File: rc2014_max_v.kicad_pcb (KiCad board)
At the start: 4 copper layers, 101.6 x 50.8 mm, 128 parts, among them J1 M3 Mounting Hole, J2 Conn_01x40, J3 Conn_01x24, J4 USB_B_Micro, J5 AVR-JTAG-10, J6 Pro Bus, J7 PMOD1, J8 PMOD2, J9 UPDI TTL, SW1 SW_Push, SW2 SW_Push, U1 TXB0108PWR, U10 ATtiny1614-SS, U11 5M1270ZT144C5N, U12 93LC46BT-I/OT, U13 IS61LV5128AL-10TLI, U14 Si5351A-B-GT, U15 TXB0108PWR, U16 TXB0108PWR, U18 MIC5356-SGYMME, U2 TXB0108PWR, U3 TXB0108PWR, U4 TXB0108PWR, U5 TXB0108PWR, U6 TXB0108PWR, U7 TXB0108PWR, U8 FT2232H, U9 TPD2EUSB30, X1 KC5032K12.0000C10E00, Y1 25MHZ 8PF

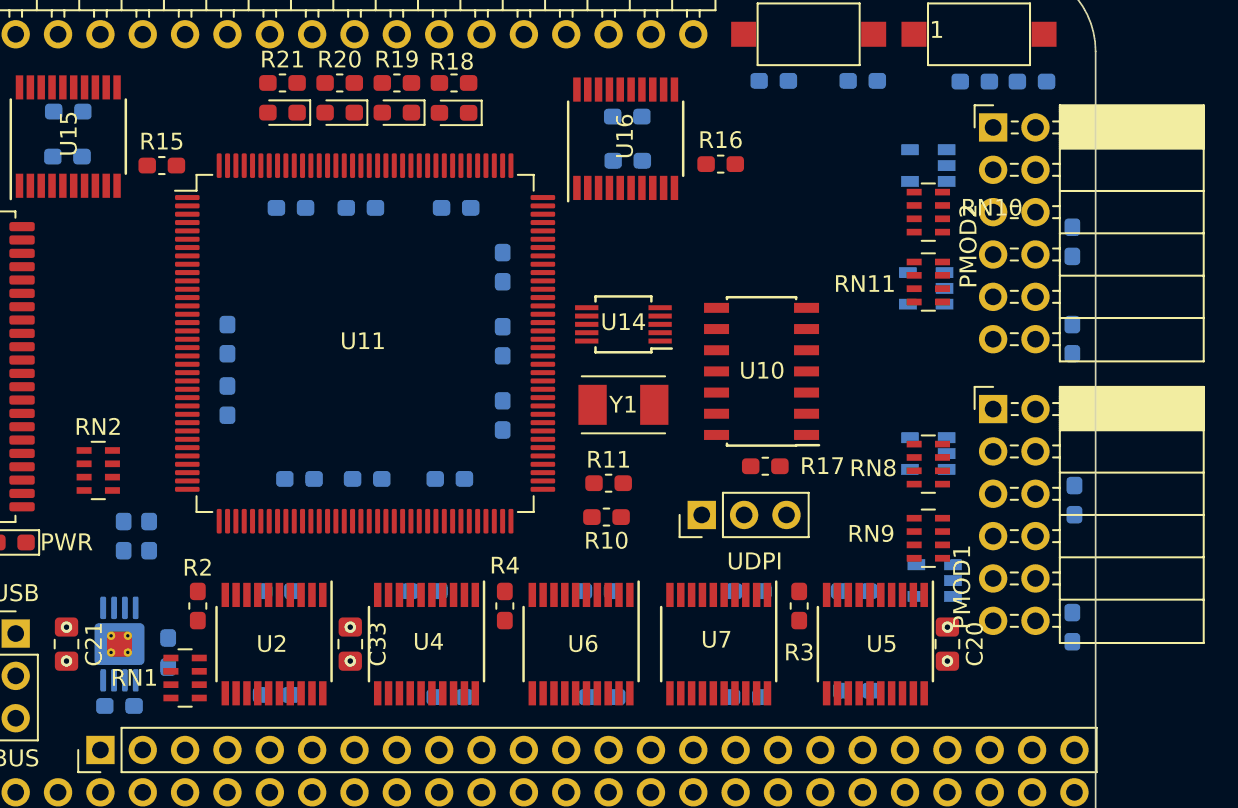
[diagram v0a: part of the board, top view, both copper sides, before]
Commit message: formatting and layer stitching
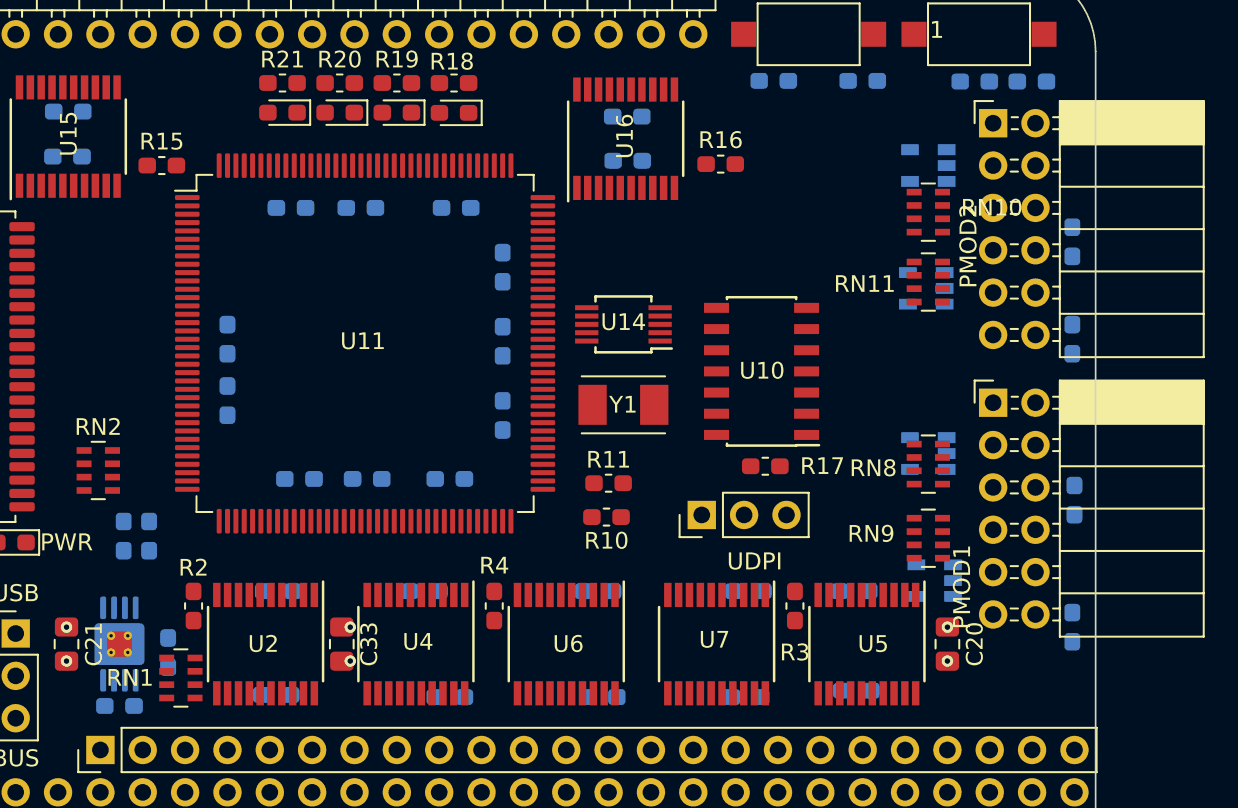
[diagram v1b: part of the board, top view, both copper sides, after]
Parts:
- moved U6 0.89 mm to (145.3, 117.3)
- moved U4 0.64 mm to (136.3, 117.3)
- moved R4 0.63 mm to (141.0, 115.1)
- moved C33 0.51 mm to (131.8, 117.3)
- moved U5 0.51 mm to (163.3, 117.3)
- moved U2 0.51 mm to (127.3, 117.3)
- moved J7 0.38 mm to (173.0, 102.9)
- moved R3 0.25 mm to (159.0, 115.1)
- moved J8 0.25 mm to (173.0, 86.1)
- moved R2 0.25 mm to (122.9, 115.1)
- moved RN1 0.25 mm to (122.2, 119.4)
- moved U7 0.13 mm to (154.3, 117.3)
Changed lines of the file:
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@@
   (page A4)
   (layers
-    (0 F.Cu signal)
-    (1 In1.Cu power hide)
+    (0 F.Cu signal hide)
+    (1 In1.Cu power)
     (2 In2.Cu power hide)
     (31 B.Cu signal)
@@
     (aux_axis_origin 0 0)
     (grid_origin 75.438 127.508)
-    (visible_elements FFFFFF7F)
+    (visible_elements FFFFF77F)
     (pcbplotparams
       (layerselection 0x010f0_ffffffff)
@@
     (add_net CLK)
     (add_net CLK2)
-    (add_net CLK2_F)
     (add_net CLK_100Mhz)
     (add_net CLK_1Mhz)
@@
     (add_net "Net-(D13-Pad4)")
     (add_net "Net-(D13-Pad5)")
-    (add_net "Net-(J2-Pad37)")
-    (add_net "Net-(J2-Pad38)")
-    (add_net "Net-(J2-Pad39)")
-    (add_net "Net-(J2-Pad40)")
-    (add_net "Net-(J3-Pad21)")
-    (add_net "Net-(J3-Pad22)")
-    (add_net "Net-(J3-Pad23)")
-    (add_net "Net-(J3-Pad24)")
     (add_net "Net-(J4-Pad2)")
     (add_net "Net-(J4-Pad3)")
-    (add_net "Net-(J5-Pad7)")
-    (add_net "Net-(J5-Pad8)")
     (add_net "Net-(LED1-Pad2)")
     (add_net "Net-(LED2-Pad2)")
@@
     (add_net "Net-(RN2-Pad3)")
     (add_net "Net-(RN2-Pad4)")
-    (add_net "Net-(RN3-Pad4)")
-    (add_net "Net-(RN3-Pad5)")
     (add_net "Net-(RN4-Pad1)")
     (add_net "Net-(RN4-Pad2)")
-    (add_net "Net-(RN4-Pad4)")
-    (add_net "Net-(RN5-Pad4)")
-    (add_net "Net-(U10-Pad11)")
-    (add_net "Net-(U10-Pad12)")
-    (add_net "Net-(U10-Pad13)")
-    (add_net "Net-(U10-Pad2)")
-    (add_net "Net-(U10-Pad3)")
-    (add_net "Net-(U10-Pad4)")
-    (add_net "Net-(U10-Pad5)")
-    (add_net "Net-(U10-Pad6)")
-    (add_net "Net-(U10-Pad7)")
-    (add_net "Net-(U11-Pad106)")
-    (add_net "Net-(U11-Pad119)")
-    (add_net "Net-(U11-Pad120)")
-    (add_net "Net-(U11-Pad121)")
-    (add_net "Net-(U11-Pad122)")
-    (add_net "Net-(U11-Pad129)")
-    (add_net "Net-(U11-Pad130)")
-    (add_net "Net-(U11-Pad131)")
-    (add_net "Net-(U11-Pad132)")
-    (add_net "Net-(U11-Pad133)")
-    (add_net "Net-(U11-Pad32)")
-    (add_net "Net-(U11-Pad72)")
-    (add_net "Net-(U13-Pad1)")
-    (add_net "Net-(U13-Pad2)")
-    (add_net "Net-(U13-Pad21)")
-    (add_net "Net-(U13-Pad22)")
-    (add_net "Net-(U13-Pad23)")
-    (add_net "Net-(U13-Pad24)")
-    (add_net "Net-(U13-Pad25)")
-    (add_net "Net-(U13-Pad39)")
-    (add_net "Net-(U13-Pad40)")
-    (add_net "Net-(U13-Pad41)")
-    (add_net "Net-(U13-Pad42)")
-    (add_net "Net-(U13-Pad43)")
-    (add_net "Net-(U13-Pad44)")
     (add_net "Net-(U14-Pad2)")
     (add_net "Net-(U14-Pad3)")
-    (add_net "Net-(U18-Pad3)")
-    (add_net "Net-(U18-Pad6)")
     (add_net "Net-(U8-Pad2)")
-    (add_net "Net-(U8-Pad21)")
-    (add_net "Net-(U8-Pad22)")
-    (add_net "Net-(U8-Pad23)")
-    (add_net "Net-(U8-Pad24)")
-    (add_net "Net-(U8-Pad26)")
-    (add_net "Net-(U8-Pad27)")
-    (add_net "Net-(U8-Pad28)")
-    (add_net "Net-(U8-Pad29)")
-    (add_net "Net-(U8-Pad3)")
-    (add_net "Net-(U8-Pad30)")
-    (add_net "Net-(U8-Pad32)")
-    (add_net "Net-(U8-Pad33)")
-    (add_net "Net-(U8-Pad34)")
-    (add_net "Net-(U8-Pad36)")
-    (add_net "Net-(U8-Pad38)")
-    (add_net "Net-(U8-Pad39)")
-    (add_net "Net-(U8-Pad40)")
-    (add_net "Net-(U8-Pad41)")
-    (add_net "Net-(U8-Pad43)")
-    (add_net "Net-(U8-Pad44)")
-    (add_net "Net-(U8-Pad45)")
-    (add_net "Net-(U8-Pad46)")
-    (add_net "Net-(U8-Pad48)")
-    (add_net "Net-(U8-Pad49)")
-    (add_net "Net-(U8-Pad50)")
-    (add_net "Net-(U8-Pad52)")
-    (add_net "Net-(U8-Pad53)")
-    (add_net "Net-(U8-Pad54)")
-    (add_net "Net-(U8-Pad55)")
-    (add_net "Net-(U8-Pad57)")
-    (add_net "Net-(U8-Pad58)")
-    (add_net "Net-(U8-Pad59)")
     (add_net OE_A)
     (add_net OE_C)
@@
   )
   (module Capacitor_SMD:C_0805_2012Metric_Pad1.15x1.40mm_HandSolder (layer F.Cu)
-    (at 132.334 117.348 270)
+    (at 131.826 117.348 270)
     (descr "Capacitor SMD 0805 (2012 Metric), square (rectangular) end terminal, IPC_7351 nominal with elongated pad for handsoldering. (Body size source: https://docs.google.com/spreadsheets/d/1BsfQQcO9C6DZCsRaXUlFlo91Tg2WpOkGARC1WS5S8t0/edit?usp=sharing), generated with kicad-footprint-generator")
     (tags "capacitor handsolder")
@@
   )
   (module Resistor_SMD:R_0603_1608Metric_Pad1.05x0.95mm_HandSolder (layer F.Cu)
-    (at 159.258 115.062 90)
+    (at 159.004 115.062 90)
     (descr "Resistor SMD 0603 (1608 Metric), square (rectangular) end terminal, IPC_7351 nominal with elongated pad for handsoldering. (Body size source: http://www.tortai-tech.com/upload/download/2011102023233369053.pdf), generated with kicad-footprint-generator")
     (tags "resistor handsolder")
@@
   )
   (module Resistor_SMD:R_0603_1608Metric_Pad1.05x0.95mm_HandSolder (layer F.Cu)
-    (at 141.605 115.062 90)
+    (at 140.97 115.062 90)
     (descr "Resistor SMD 0603 (1608 Metric), square (rectangular) end terminal, IPC_7351 nominal with elongated pad for handsoldering. (Body size source: http://www.tortai-tech.com/upload/download/2011102023233369053.pdf), generated with kicad-footprint-generator")
     (tags "resistor handsolder")
@@
   )
   (module Resistor_SMD:R_0603_1608Metric_Pad1.05x0.95mm_HandSolder (layer F.Cu)
-    (at 123.19 115.062 90)
+    (at 122.936 115.062 90)
     (descr "Resistor SMD 0603 (1608 Metric), square (rectangular) end terminal, IPC_7351 nominal with elongated pad for handsoldering. (Body size source: http://www.tortai-tech.com/upload/download/2011102023233369053.pdf), generated with kicad-footprint-generator")
     (tags "resistor handsolder")
@@
   )
   (module Resistor_SMD:R_Array_Concave_4x0603 (layer F.Cu)
-    (at 122.428 119.38)
+    (at 122.174 119.38)
     (descr "Thick Film Chip Resistor Array, Wave soldering, Vishay CRA06P (see cra06p.pdf)")
     (tags "resistor array")
@@
   )
   (module Package_SO:TSSOP-20_4.4x6.5mm_P0.65mm (layer F.Cu)
-    (at 154.432 117.348 270)
+    (at 154.305 117.348 270)
     (descr "20-Lead Plastic Thin Shrink Small Outline (ST)-4.4 mm Body [TSSOP] (see Microchip Packaging Specification 00000049BS.pdf)")
     (tags "SSOP 0.65")
@@
   )
   (module Package_SO:TSSOP-20_4.4x6.5mm_P0.65mm (layer F.Cu)
-    (at 163.83 117.348 270)
+    (at 163.322 117.348 270)
     (descr "20-Lead Plastic Thin Shrink Small Outline (ST)-4.4 mm Body [TSSOP] (see Microchip Packaging Specification 00000049BS.pdf)")
     (tags "SSOP 0.65")
@@
   )
   (module Package_SO:TSSOP-20_4.4x6.5mm_P0.65mm (layer F.Cu)
-    (at 146.177 117.348 270)
+    (at 145.288 117.348 270)
     (descr "20-Lead Plastic Thin Shrink Small Outline (ST)-4.4 mm Body [TSSOP] (see Microchip Packaging Specification 00000049BS.pdf)")
     (tags "SSOP 0.65")
@@
   )
   (module Package_SO:TSSOP-20_4.4x6.5mm_P0.65mm (layer F.Cu)
-    (at 136.906 117.348 270)
+    (at 136.271 117.348 270)
     (descr "20-Lead Plastic Thin Shrink Small Outline (ST)-4.4 mm Body [TSSOP] (see Microchip Packaging Specification 00000049BS.pdf)")
     (tags "SSOP 0.65")
@@
   )
   (module Package_SO:TSSOP-20_4.4x6.5mm_P0.65mm (layer F.Cu)
-    (at 127.762 117.348 270)
+    (at 127.254 117.348 270)
     (descr "20-Lead Plastic Thin Shrink Small Outline (ST)-4.4 mm Body [TSSOP] (see Microchip Packaging Specification 00000049BS.pdf)")
     (tags "SSOP 0.65")
@@
   )
   (module Connector_PinSocket_2.54mm:PinSocket_2x06_P2.54mm_Horizontal (layer F.Cu)
-    (at 172.974 86.36)
+    (at 172.974 86.106)
     (descr "Through hole angled socket strip, 2x06, 2.54mm pitch, 8.51mm socket length, double cols (from Kicad 4.0.7), script generated")
     (tags "Through hole angled socket strip THT 2x06 2.54mm double row")
@@
   )
   (module Connector_PinSocket_2.54mm:PinSocket_2x06_P2.54mm_Horizontal (layer F.Cu)
-    (at 172.974 103.251)
+    (at 172.974 102.87)
     (descr "Through hole angled socket strip, 2x06, 2.54mm pitch, 8.51mm socket length, double cols (from Kicad 4.0.7), script generated")
     (tags "Through hole angled socket strip THT 2x06 2.54mm double row")
@@
   (gr_line (start 177.038 127.508) (end 75.438 127.508) (layer Edge.Cuts) (width 0.1))
   (gr_line (start 75.438 127.508) (end 75.438 91.948) (layer Edge.Cuts) (width 0.1))
-  (via (at 84.328 116.332) (size 0.6858) (drill 0.3302) (layers F.Cu B.Cu) (net 198))
   (via (at 84.328 118.364) (size 0.6858) (drill 0.3302) (layers F.Cu B.Cu) (net 1))
-  (via (at 115.316 116.332) (size 0.6858) (drill 0.3302) (layers F.Cu B.Cu) (net 198))
   (via (at 115.316 118.364) (size 0.6858) (drill 0.3302) (layers F.Cu B.Cu) (net 1))
-  (via (at 168.148 116.332) (size 0.6858) (drill 0.3302) (layers F.Cu B.Cu) (net 198))
   (via (at 168.148 118.364) (size 0.6858) (drill 0.3302) (layers F.Cu B.Cu) (net 1))
-  (via (at 132.334 116.332) (size 0.6858) (drill 0.3302) (layers F.Cu B.Cu) (net 198))
   (via (at 132.334 118.364) (size 0.6858) (drill 0.3302) (layers F.Cu B.Cu) (net 1))
+  (via (at 84.328 116.332) (size 0.6858) (drill 0.3302) (layers F.Cu B.Cu) (net 198))
+  (via (at 115.316 116.332) (size 0.6858) (drill 0.3302) (layers F.Cu B.Cu) (net 198))
+  (via (at 168.148 116.332) (size 0.6858) (drill 0.3302) (layers F.Cu B.Cu) (net 198))
+  (via (at 132.334 116.332) (size 0.6858) (drill 0.3302) (layers F.Cu B.Cu) (net 198))
   (zone (net 2) (net_name GND) (layer In2.Cu) (hatch edge 0.508)
     (connect_pads (clearance 0.508))
